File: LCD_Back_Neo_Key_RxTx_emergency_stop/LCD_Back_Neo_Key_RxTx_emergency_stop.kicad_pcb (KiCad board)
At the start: 2 copper layers, 104.2 x 101.5 mm, 21 parts, among them J1 Screw_Terminal_01x09, J2 Conn_01x20_Female, J3 Conn_01x08_Male_KeyPad, J4 Display_support_pin, J5 Display_support_pin, J6 Screw_Terminal_01x05, K1 FINDER-34.51, K2 FINDER-34.51, K3 FINDER-34.51, Q1 BC337, Q2 2N2222, U1 DC-DC_Stepdown-Zimprich

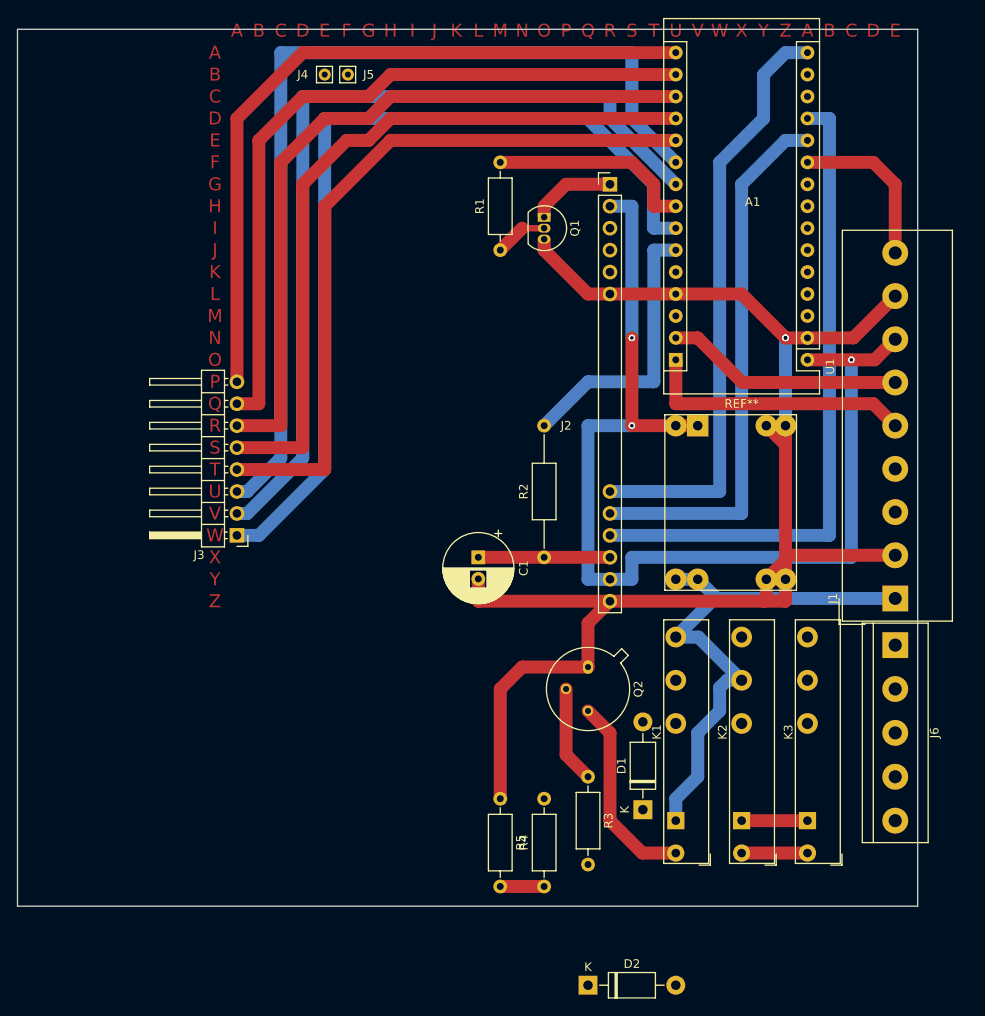
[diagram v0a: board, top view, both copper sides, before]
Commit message: remove ABCCDEF....
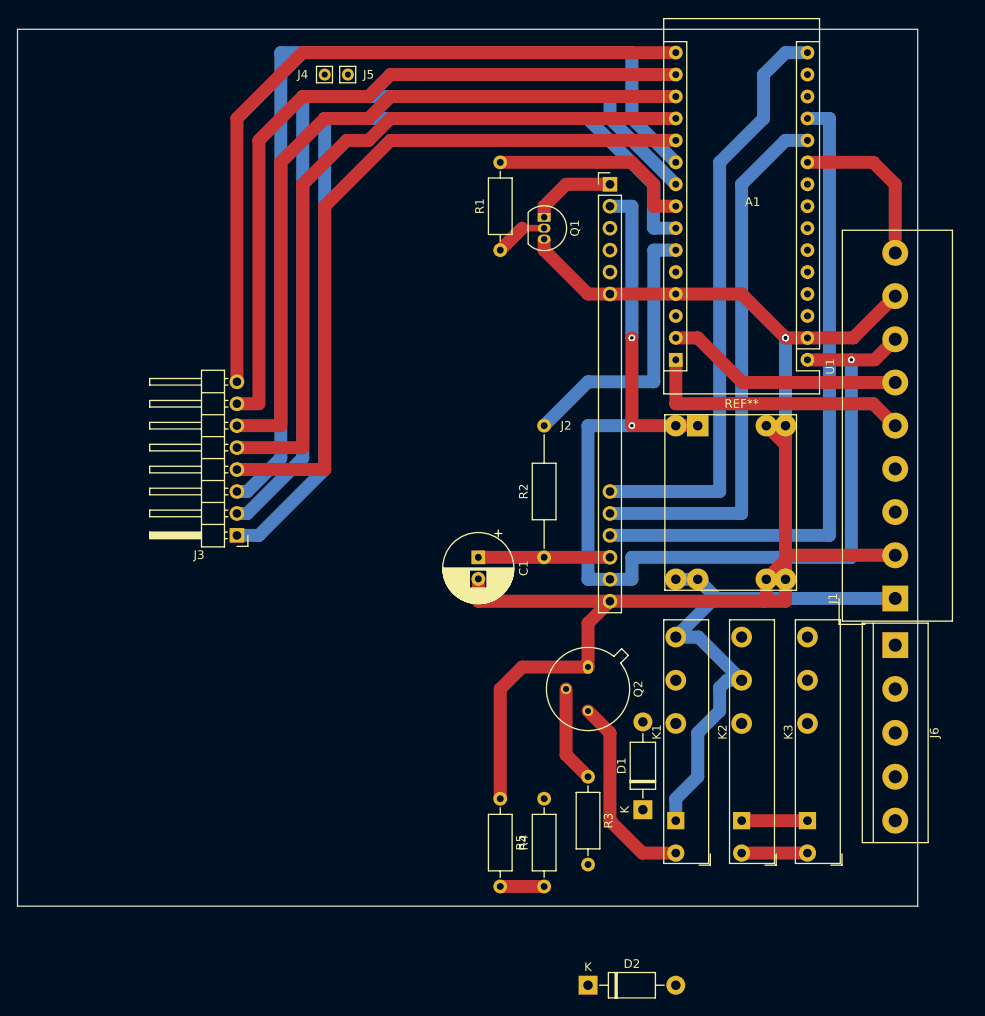
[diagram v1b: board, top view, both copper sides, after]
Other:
- board text removed: "A"
- board text removed: "B"
- board text removed: "C"
- board text removed: "D"
- board text removed: "E"
- board text removed: "F"
- board text removed: "G"
- board text removed: "H"
- board text removed: "I"
- board text removed: "J"
- board text removed: "K"
- board text removed: "L"
- board text removed: "M"
- board text removed: "N"
- board text removed: "O"
- board text removed: "P"
- board text removed: "Q"
- board text removed: "R"
- board text removed: "S"
- board text removed: "T"
- board text removed: "U"
- board text removed: "V"
- board text removed: "W"
- board text removed: "X"
- board text removed: "Y"
- board text removed: "Z"
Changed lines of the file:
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@@
-(kicad_pcb (version 20171130) (host pcbnew "(5.1.0-9-gc61ec8ee3)")
+(kicad_pcb (version 20171130) (host pcbnew "(5.1.0-13-ge6234d50d)")
   (general
     (thickness 1.6)
-    (drawings 61)
+    (drawings 4)
     (tracks 161)
     (zones 0)
@@
   (gr_line (start 208.34 32.86) (end 208.34 134.36) (layer Edge.Cuts) (width 0.05))
   (gr_line (start 104.14 134.36) (end 208.34 134.36) (layer Edge.Cuts) (width 0.05))
-  (gr_text C (at 200.66 33.02) (layer F.Cu)
-    (effects (font (size 1.5 1.5) (thickness 0.3)))
-  )
-  (gr_text D (at 203.2 33.02) (layer F.Cu)
-    (effects (font (size 1.5 1.5) (thickness 0.3)))
-  )
-  (gr_text B (at 198.12 33.02) (layer F.Cu)
-    (effects (font (size 1.5 1.5) (thickness 0.3)))
-  )
-  (gr_text A (at 195.58 33.02) (layer F.Cu)
-    (effects (font (size 1.5 1.5) (thickness 0.3)))
-  )
-  (gr_text E (at 205.74 33.02) (layer F.Cu)
-    (effects (font (size 1.5 1.5) (thickness 0.3)))
-  )
-  (gr_text N (at 162.56 33.02) (layer F.Cu)
-    (effects (font (size 1.5 1.5) (thickness 0.3)))
-  )
-  (gr_text M (at 160.02 33.02) (layer F.Cu)
-    (effects (font (size 1.5 1.5) (thickness 0.3)))
-  )
-  (gr_text Z (at 193.04 33.02) (layer F.Cu)
-    (effects (font (size 1.5 1.5) (thickness 0.3)))
-  )
-  (gr_text Y (at 190.5 33.02) (layer F.Cu)
-    (effects (font (size 1.5 1.5) (thickness 0.3)))
-  )
-  (gr_text X (at 187.96 33.02) (layer F.Cu)
-    (effects (font (size 1.5 1.5) (thickness 0.3)))
-  )
-  (gr_text W (at 185.42 33.02) (layer F.Cu)
-    (effects (font (size 1.5 1.5) (thickness 0.3)))
-  )
-  (gr_text V (at 182.88 33.02) (layer F.Cu)
-    (effects (font (size 1.5 1.5) (thickness 0.3)))
-  )
-  (gr_text U (at 180.34 33.02) (layer F.Cu)
-    (effects (font (size 1.5 1.5) (thickness 0.3)))
-  )
-  (gr_text T (at 177.8 33.02) (layer F.Cu)
-    (effects (font (size 1.5 1.5) (thickness 0.3)))
-  )
-  (gr_text S (at 175.26 33.02) (layer F.Cu)
-    (effects (font (size 1.5 1.5) (thickness 0.3)))
-  )
-  (gr_text R (at 172.72 33.02) (layer F.Cu)
-    (effects (font (size 1.5 1.5) (thickness 0.3)))
-  )
-  (gr_text Q (at 170.18 33.02) (layer F.Cu)
-    (effects (font (size 1.5 1.5) (thickness 0.3)))
-  )
-  (gr_text P (at 167.64 33.02) (layer F.Cu)
-    (effects (font (size 1.5 1.5) (thickness 0.3)))
-  )
-  (gr_text O (at 165.1 33.02) (layer F.Cu)
-    (effects (font (size 1.5 1.5) (thickness 0.3)))
-  )
-  (gr_text L (at 157.48 33.02) (layer F.Cu)
-    (effects (font (size 1.5 1.5) (thickness 0.3)))
-  )
-  (gr_text K (at 154.94 33.02) (layer F.Cu)
-    (effects (font (size 1.5 1.5) (thickness 0.3)))
-  )
-  (gr_text I (at 149.86 33.02) (layer F.Cu)
-    (effects (font (size 1.5 1.5) (thickness 0.3)))
-  )
-  (gr_text J (at 152.4 33.02) (layer F.Cu)
-    (effects (font (size 1.5 1.5) (thickness 0.3)))
-  )
-  (gr_text H (at 147.32 33.02) (layer F.Cu)
-    (effects (font (size 1.5 1.5) (thickness 0.3)))
-  )
-  (gr_text G (at 144.78 33.02) (layer F.Cu)
-    (effects (font (size 1.5 1.5) (thickness 0.3)))
-  )
-  (gr_text F (at 142.24 33.02) (layer F.Cu)
-    (effects (font (size 1.5 1.5) (thickness 0.3)))
-  )
-  (gr_text E (at 139.7 33.02) (layer F.Cu)
-    (effects (font (size 1.5 1.5) (thickness 0.3)))
-  )
-  (gr_text D (at 137.16 33.02) (layer F.Cu)
-    (effects (font (size 1.5 1.5) (thickness 0.3)))
-  )
-  (gr_text C (at 134.62 33.02) (layer F.Cu)
-    (effects (font (size 1.5 1.5) (thickness 0.3)))
-  )
-  (gr_text B (at 132.08 33.02) (layer F.Cu)
-    (effects (font (size 1.5 1.5) (thickness 0.3)))
-  )
-  (gr_text A (at 129.54 33.02) (layer F.Cu)
-    (effects (font (size 1.5 1.5) (thickness 0.3)))
-  )
-  (gr_text A (at 127 35.56) (layer F.Cu)
-    (effects (font (size 1.5 1.5) (thickness 0.3)))
-  )
-  (gr_text B (at 127 38.1) (layer F.Cu)
-    (effects (font (size 1.5 1.5) (thickness 0.3)))
-  )
-  (gr_text C (at 127 40.64) (layer F.Cu)
-    (effects (font (size 1.5 1.5) (thickness 0.3)))
-  )
-  (gr_text D (at 127 43.18) (layer F.Cu)
-    (effects (font (size 1.5 1.5) (thickness 0.3)))
-  )
-  (gr_text E (at 127 45.72) (layer F.Cu)
-    (effects (font (size 1.5 1.5) (thickness 0.3)))
-  )
-  (gr_text F (at 127 48.26) (layer F.Cu)
-    (effects (font (size 1.5 1.5) (thickness 0.3)))
-  )
-  (gr_text G (at 127 50.8) (layer F.Cu)
-    (effects (font (size 1.5 1.5) (thickness 0.3)))
-  )
-  (gr_text H (at 127 53.34) (layer F.Cu)
-    (effects (font (size 1.5 1.5) (thickness 0.3)))
-  )
-  (gr_text I (at 127 55.88) (layer F.Cu)
-    (effects (font (size 1.5 1.5) (thickness 0.3)))
-  )
-  (gr_text J (at 127 58.42) (layer F.Cu)
-    (effects (font (size 1.5 1.5) (thickness 0.3)))
-  )
-  (gr_text K (at 127 60.96) (layer F.Cu)
-    (effects (font (size 1.5 1.5) (thickness 0.3)))
-  )
-  (gr_text L (at 127 63.5) (layer F.Cu)
-    (effects (font (size 1.5 1.5) (thickness 0.3)))
-  )
-  (gr_text M (at 127 66.04) (layer F.Cu)
-    (effects (font (size 1.5 1.5) (thickness 0.3)))
-  )
-  (gr_text N (at 127 68.58) (layer F.Cu)
-    (effects (font (size 1.5 1.5) (thickness 0.3)))
-  )
-  (gr_text O (at 127 71.12) (layer F.Cu)
-    (effects (font (size 1.5 1.5) (thickness 0.3)))
-  )
-  (gr_text P (at 127 73.66) (layer F.Cu)
-    (effects (font (size 1.5 1.5) (thickness 0.3)))
-  )
-  (gr_text Q (at 127 76.2) (layer F.Cu)
-    (effects (font (size 1.5 1.5) (thickness 0.3)))
-  )
-  (gr_text R (at 127 78.74) (layer F.Cu)
-    (effects (font (size 1.5 1.5) (thickness 0.3)))
-  )
-  (gr_text S (at 127 81.28) (layer F.Cu)
-    (effects (font (size 1.5 1.5) (thickness 0.3)))
-  )
-  (gr_text T (at 127 83.82) (layer F.Cu)
-    (effects (font (size 1.5 1.5) (thickness 0.3)))
-  )
-  (gr_text U (at 127 86.36) (layer F.Cu)
-    (effects (font (size 1.5 1.5) (thickness 0.3)))
-  )
-  (gr_text V (at 127 88.9) (layer F.Cu)
-    (effects (font (size 1.5 1.5) (thickness 0.3)))
-  )
-  (gr_text W (at 127 91.44) (layer F.Cu)
-    (effects (font (size 1.5 1.5) (thickness 0.3)))
-  )
-  (gr_text X (at 127 93.98) (layer F.Cu)
-    (effects (font (size 1.5 1.5) (thickness 0.3)))
-  )
-  (gr_text Y (at 127 96.52) (layer F.Cu)
-    (effects (font (size 1.5 1.5) (thickness 0.3)))
-  )
-  (gr_text Z (at 127 99.06) (layer F.Cu)
-    (effects (font (size 1.5 1.5) (thickness 0.3)))
-  )
   (segment (start 180.34 76.2) (end 203.2 76.2) (width 1.5) (layer F.Cu) (net 1))
   (segment (start 203.2 76.2) (end 205.74 78.74) (width 1.5) (layer F.Cu) (net 1))
@@
   (segment (start 180.34 121.92) (end 180.34 124.46) (width 1.5) (layer B.Cu) (net 36))
   (segment (start 182.88 119.38) (end 180.34 121.92) (width 1.5) (layer B.Cu) (net 36))
-  (segment (start 187.96 124.46) (end 195.58 124.46) (width 1.5) (layer F.Cu) (net 48))
-  (segment (start 176.47 128.21) (end 180.34 128.21) (width 1.5) (layer F.Cu) (net 47))
-  (segment (start 172.72 124.46) (end 176.47 128.21) (width 1.5) (layer F.Cu) (net 47))
-  (segment (start 170.18 111.76) (end 172.72 114.3) (width 1.5) (layer F.Cu) (net 47))
-  (segment (start 172.72 114.3) (end 172.72 124.46) (width 1.5) (layer F.Cu) (net 47))
-  (segment (start 187.96 128.21) (end 195.58 128.21) (width 1.5) (layer F.Cu) (net 49))
   (segment (start 167.64 109.22) (end 167.64 116.84) (width 1.5) (layer F.Cu) (net 42))
   (segment (start 167.64 116.84) (end 170.18 119.38) (width 1.5) (layer F.Cu) (net 42))
@@
   (segment (start 205.74 50.8) (end 205.74 57.15) (width 1.5) (layer F.Cu) (net 43))
   (segment (start 160.02 132.08) (end 165.1 132.08) (width 1.5) (layer F.Cu) (net 46))
+  (segment (start 176.47 128.21) (end 180.34 128.21) (width 1.5) (layer F.Cu) (net 47))
+  (segment (start 172.72 124.46) (end 176.47 128.21) (width 1.5) (layer F.Cu) (net 47))
+  (segment (start 170.18 111.76) (end 172.72 114.3) (width 1.5) (layer F.Cu) (net 47))
+  (segment (start 172.72 114.3) (end 172.72 124.46) (width 1.5) (layer F.Cu) (net 47))
+  (segment (start 187.96 124.46) (end 195.58 124.46) (width 1.5) (layer F.Cu) (net 48))
+  (segment (start 187.96 128.21) (end 195.58 128.21) (width 1.5) (layer F.Cu) (net 49))
 )

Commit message: place screwterminal on PCB
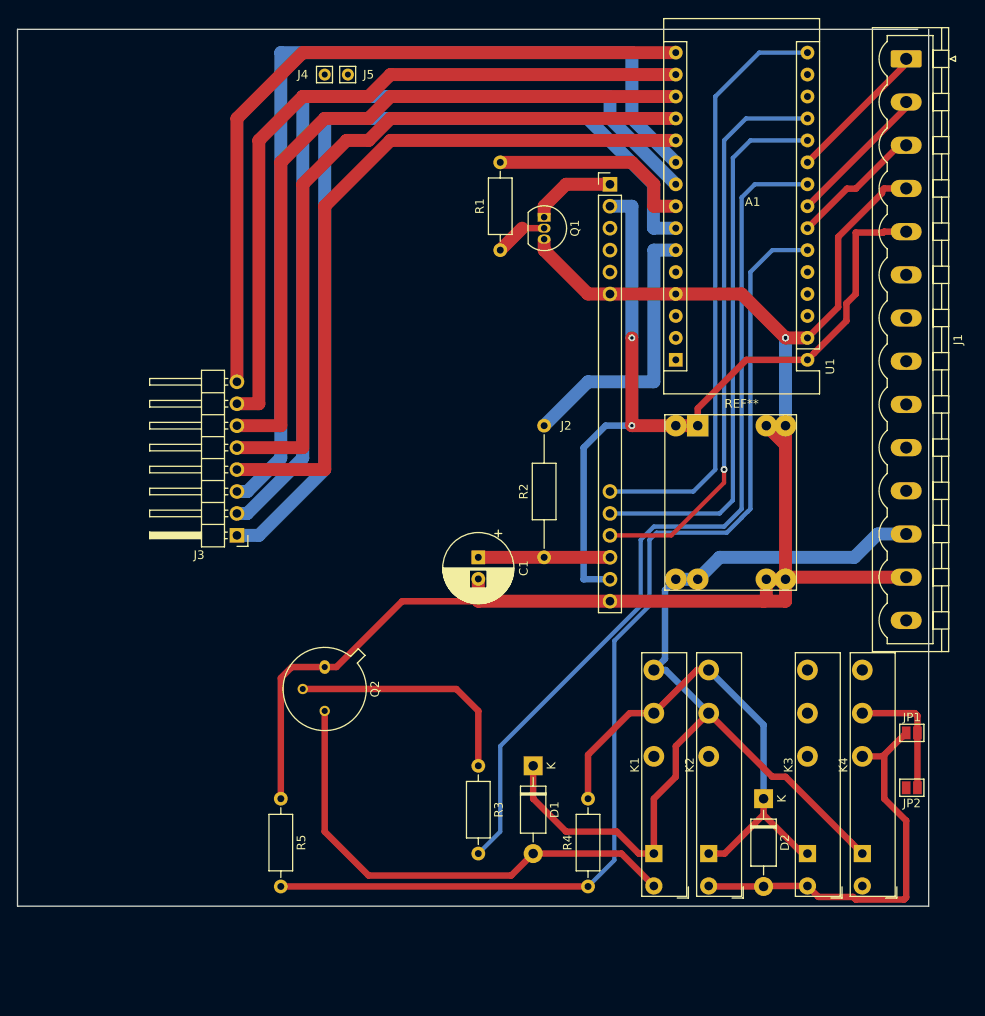
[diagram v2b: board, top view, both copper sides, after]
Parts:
- removed J6: Screw_Terminal_01x05, TerminalBlock:TerminalBlock_bornier-5_P5.08mm
- added JP1: Jumper_lon-jumper_lon, Jumper:SolderJumper-2_P1.3mm_Open_Pad1.0x1.5mm, F.Cu at (207.7, 114.3)
- added JP2: Jumper_lon-jumper_lon, Jumper:SolderJumper-2_P1.3mm_Open_Pad1.0x1.5mm, F.Cu at (207.7, 120.7)
- added K4: FINDER-34.51, Relay_THT:Relay_SPDT_Finder_34.51_Vertical, F.Cu at (201.9, 128.3)
- J1: value Screw_Terminal_01x09 -> Screw_Terminal_01x14; footprint TerminalBlock_Altech:Altech_AK300_1x09_P5.00mm_45-Degree -> Connector_Phoenix_MSTB:PhoenixContact_MSTBVA_2,5_14-G_1x14_P5.00mm_Vertical
- moved J1 62.5 mm to (207.0, 36.3), turned to 270 degrees
- moved Q2 30.5 mm to (139.7, 106.7)
- moved D2 29.6 mm to (190.5, 121.9), turned to 270 degrees
- moved R5 25.4 mm to (134.6, 121.9)
- moved D1 13.7 mm to (163.8, 118.1), turned to 270 degrees
- moved R3 12.8 mm to (157.5, 118.1)
- moved K2 5.39 mm to (184.2, 128.3)
- moved R4 5.08 mm to (170.2, 132.1)
- moved K1 4.58 mm to (177.8, 128.3)
- moved K3 3.81 mm to (195.6, 128.3)
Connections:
- J1 pad 1: VCC-24V -> Ardu_A2
- J1 pad 2: GND -> Ardu_A4
- J1 pad 3: Net-(J1-Pad3) -> Ardu_A5
- J1 pad 4: Net-(J1-Pad4) -> GND
- J1 pad 5: Net-(A1-Pad1) -> VCC-5V
- J1 pad 6: Net-(A1-Pad2) -> ScrewTerm8-EmrgencyRelay12
- J1 pad 7: VCC-5V -> ScrewTerm9-EmrgencyRelay14
- J1 pad 8: GND -> ScrewTerm10-EmrgencyRelay11
- J1 pad 9: Ardu_A2 -> ScrewTerm11-EmergencyStopSwitch1
- K3 pad 11: Net-(J6-Pad3) -> ScrewTerm10-EmrgencyRelay11
- K3 pad 12: Net-(J6-Pad1) -> ScrewTerm8-EmrgencyRelay12
- K3 pad 14: Net-(J6-Pad2) -> ScrewTerm9-EmrgencyRelay14
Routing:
- net Ardu_A6: track 5.08 -> 126.9 mm
- net Ardu_A3: track 0.00 -> 101.6 mm
- net Net-(D2-Pad1): track 7.62 -> 57.7 mm
- net VCC-24V: track 63.0 -> 112.6 mm
- net Net-(D2-Pad2): track 7.62 -> 47.4 mm
- net Net-(D1-Pad2): track 22.9 -> 56.8 mm
- net Net-(A1-Pad1): track 31.5 -> 0.00 mm
- net Net-(A1-Pad2): track 27.5 -> 0.00 mm
- net VCC-5V: track 125.4 -> 100.4 mm, vias 3 -> 2
- net GND: track 173.4 -> 190.8 mm
- net Ardu_A4: track 0.00 -> 16.8 mm
- net Net-(Q2-Pad2): track 11.2 -> 27.7 mm
- net Ardu_A5: track 0.00 -> 15.4 mm
- net ScrewTerm11-EmergencyStopSwitch1: track 0.00 -> 14.8 mm
- net Ardu_A0: track 76.2 -> 66.1 mm, vias 0 -> 1
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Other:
- board size 104.2 x 101.5 mm -> 105.5 x 101.5 mm
